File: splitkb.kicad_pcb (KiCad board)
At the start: 2 copper layers, 153 x 123.5 mm, 77 parts, among them J1 MJ-4PP-9, K1 KEYSW, SW1 SW_PUSH, SW10 SW_PUSH, SW11 SW_PUSH, SW12 SW_PUSH, SW13 SW_PUSH, SW14 SW_PUSH, SW15 SW_PUSH, SW16 SW_PUSH, SW17 SW_PUSH, SW18 SW_PUSH, SW19 SW_PUSH, SW2 SW_PUSH, SW20 SW_PUSH, SW21 SW_PUSH, SW22 SW_PUSH, SW23 SW_PUSH, SW24 SW_PUSH, SW25 SW_PUSH, SW26 SW_PUSH, SW27 SW_PUSH, SW28 SW_PUSH, SW29 SW_PUSH, SW3 SW_PUSH, SW30 SW_PUSH, SW31 SW_PUSH, SW32 SW_PUSH, SW4 SW_PUSH, SW5 SW_PUSH, SW6 SW_PUSH, SW7 SW_PUSH, SW8 SW_PUSH, SW9 SW_PUSH, U1 ProMicro

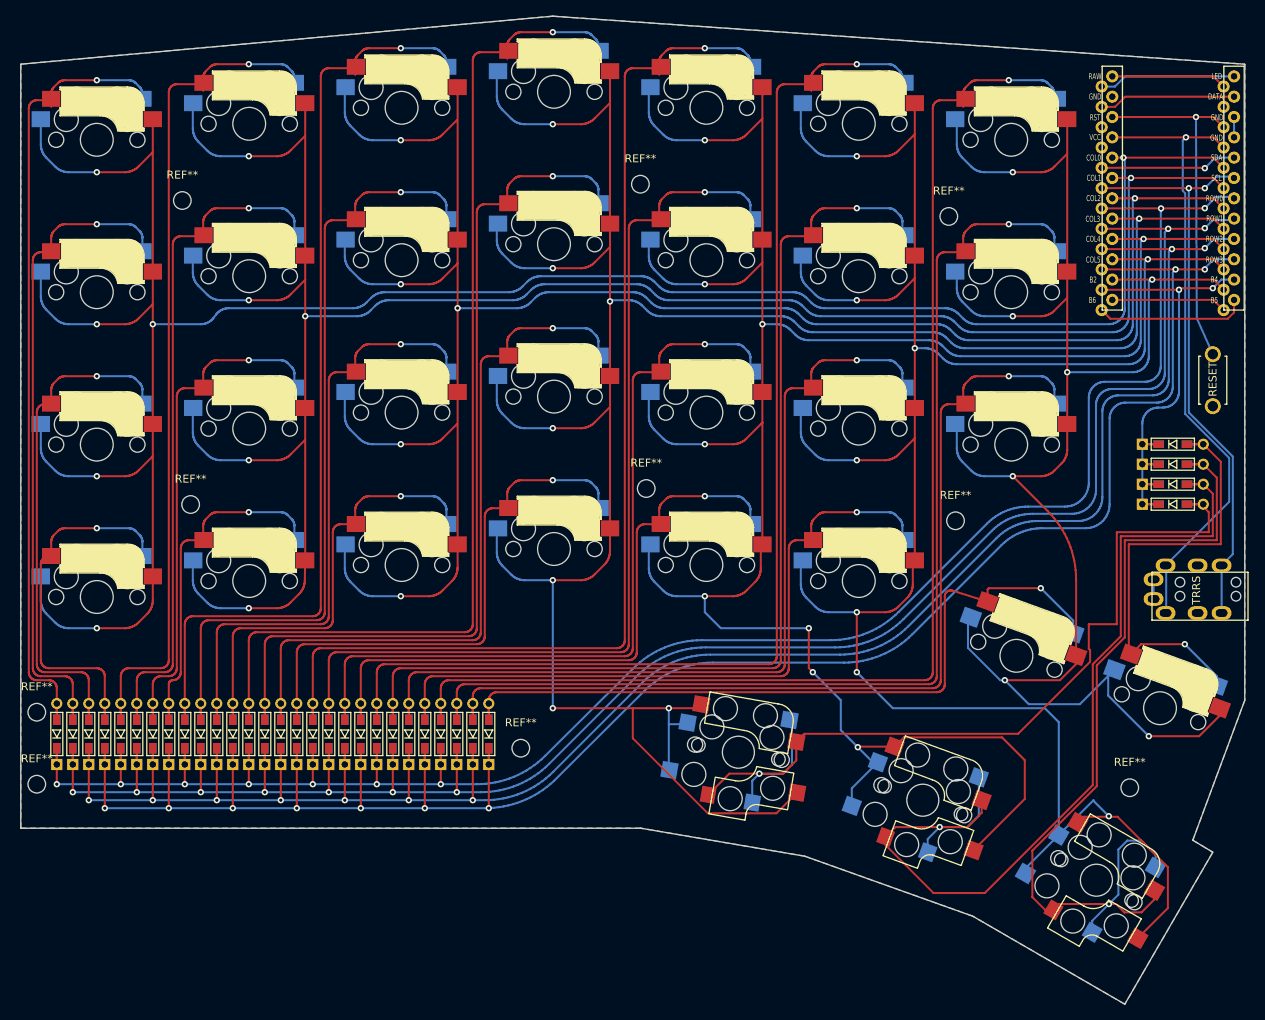
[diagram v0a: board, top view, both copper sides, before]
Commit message: positioning
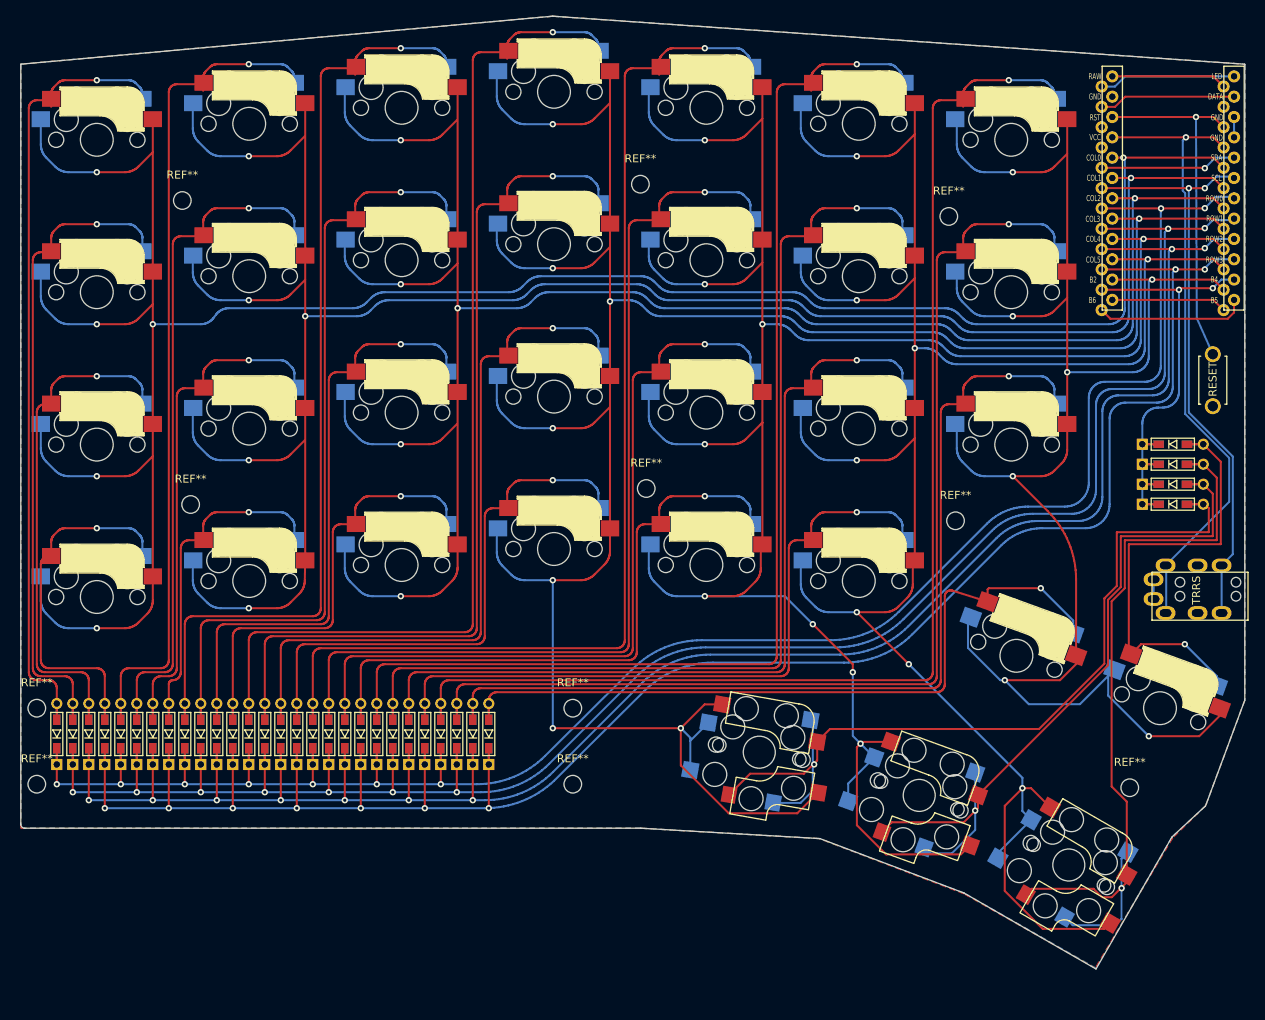
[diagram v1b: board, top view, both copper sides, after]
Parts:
- added REF**: MountingHole_2.2mm_M2, MountingHole:MountingHole_2.2mm_M2, F.Cu at (107.5, 133.5)
- moved REF** 8.20 mm to (107.5, 124.0)
- moved SW27 3.94 mm to (169.5, 143.6)
- moved SW17 2.61 mm to (130.8, 129.5)
- moved SW22 0.75 mm to (150.8, 134.9)
- moved REF** 0.50 mm to (40.5, 124.0)
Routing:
- net Net-(D22-Pad2): track 119.0 -> 92.4 mm
- net col5: track 287.2 -> 272.2 mm
- net Net-(D27-Pad2): track 112.8 -> 100.7 mm
- net col4: track 297.7 -> 289.7 mm
- net Net-(D17-Pad2): track 109.4 -> 106.7 mm
- net col3: track 312.6 -> 313.3 mm
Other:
- board size 153 x 123.5 mm -> 153 x 119.1 mm
